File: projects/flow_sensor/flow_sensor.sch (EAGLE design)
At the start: 81 parts, among them IC1 TPS61201, IC5 REG1118

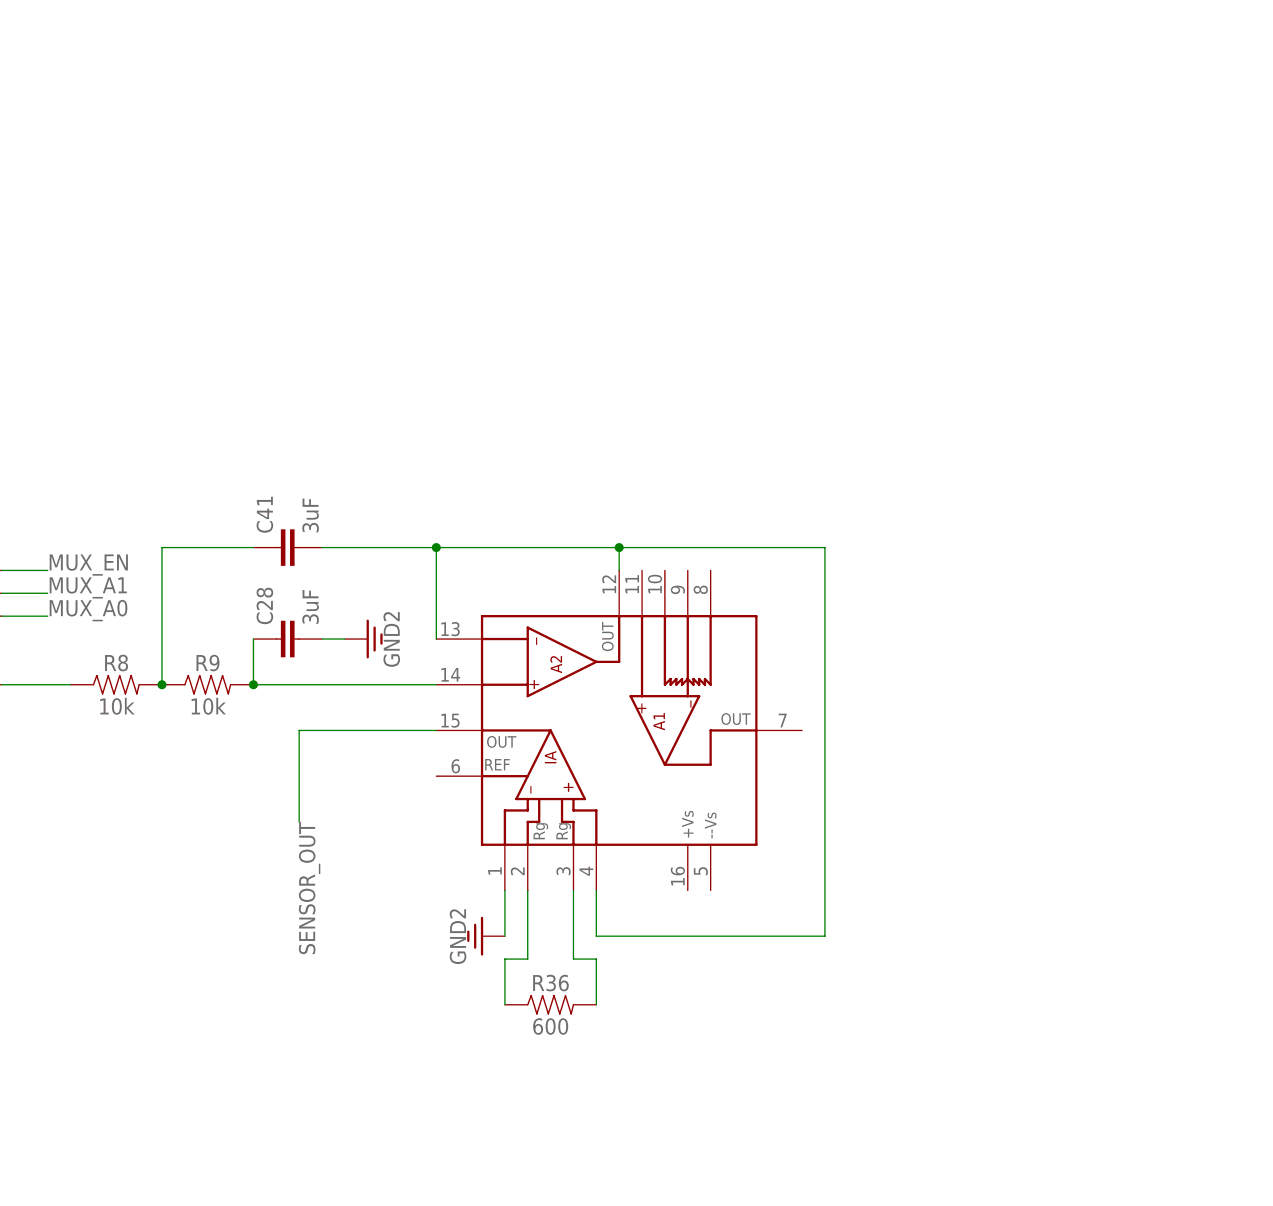
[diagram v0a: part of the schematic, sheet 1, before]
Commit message: Resubmitting work for 1/24/18
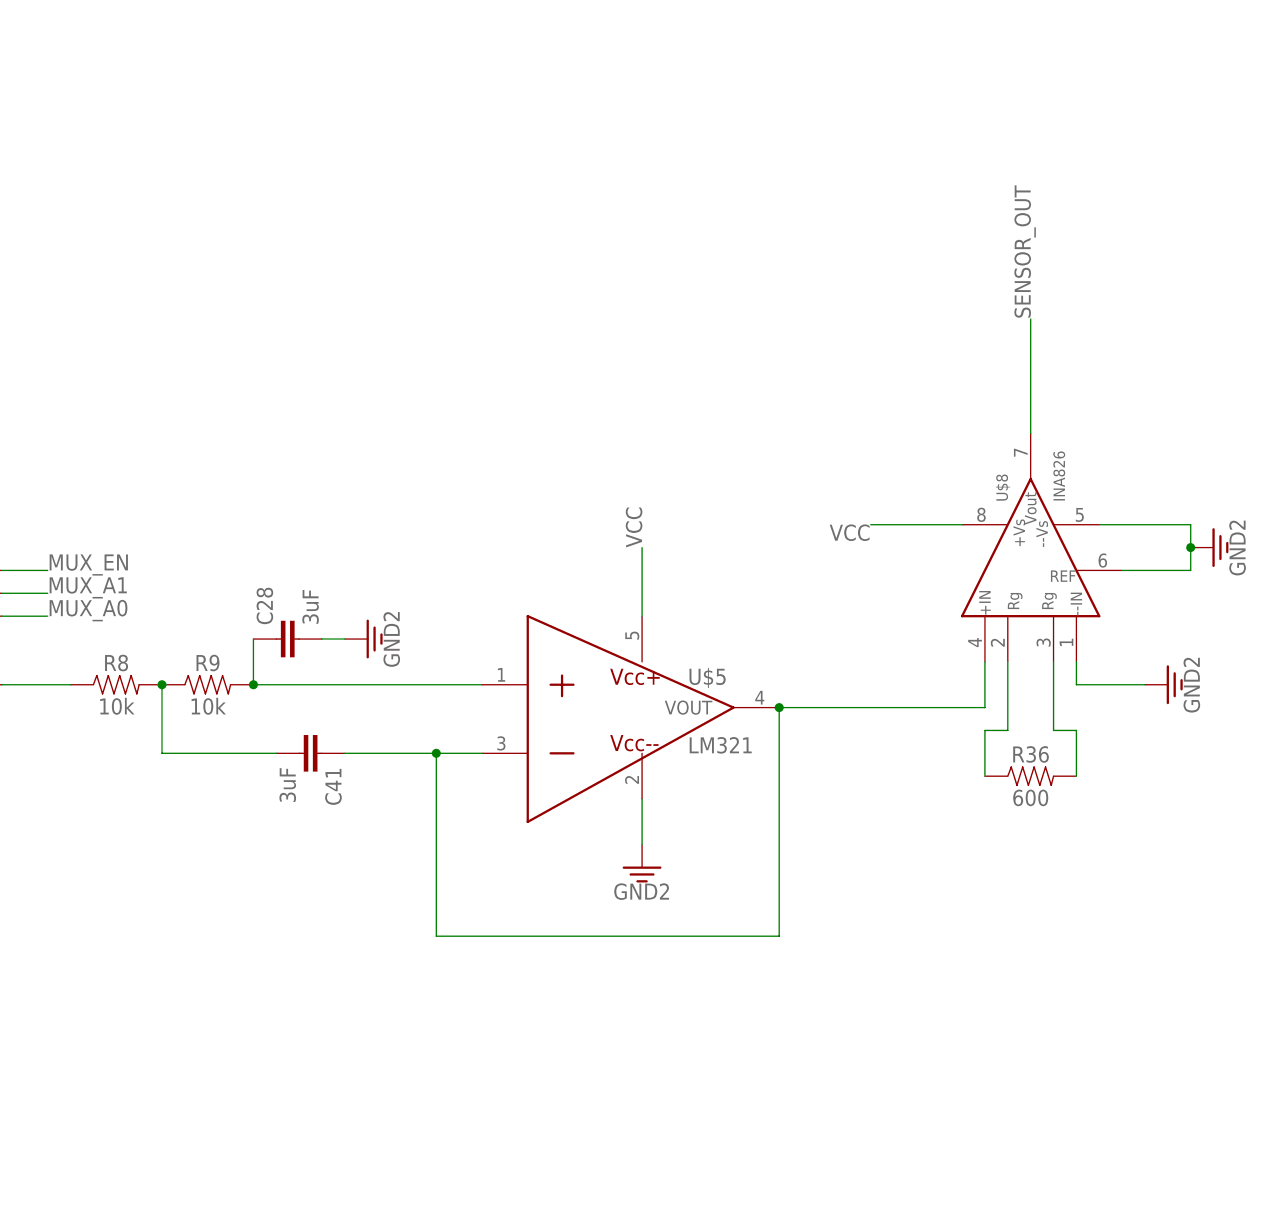
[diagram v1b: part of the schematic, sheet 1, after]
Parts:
- added U$5: LM321, my_library:LM321
- U$8: value AD8295 -> INA826; device my_library:AD8295 -> my_library:INA826
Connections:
- removed net N$35: C41.1, R8.2, R9.1
- removed net N$48: C41.2, U$8.+IN, U$8.A2-IN, U$8.A2OUT
- new net N$31: C41.1, U$5.IN-, U$5.VOUT, U$8.IN+
- new net N$36: C41.2, R8.2, R9.1
- net 3.3V: now also U$5.VCC-, U$8.IN-, U$8.REF, U$8.VS-; no longer U$8.-IN
- net N$19: now also U$5.IN+; no longer U$8.A2+IN
- net SENSOR_OUT: now also U$8.VOUT; no longer U$8.OUT
- net VCC: now also U$5.VCC+, U$8.VS+
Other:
- moved on the sheet: C41, R36
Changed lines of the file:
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@@
 <part name="U$7" library="my_library" deviceset="MAX4634" device=""/>
 <part name="GND35" library="SparkFun-PowerSymbols" deviceset="GND2" device=""/>
-<part name="U$8" library="my_library" deviceset="AD8295" device=""/>
 <part name="C41" library="SparkFun-Capacitors" deviceset="4.7UF" device="0603" value="3uF"/>
 <part name="GND36" library="SparkFun-PowerSymbols" deviceset="GND2" device=""/>
 <part name="R36" library="SparkFun-Resistors" deviceset="787OHM" device="-0603-1/10W-1%" value="600"/>
+<part name="U$5" library="my_library" deviceset="LM321" device=""/>
+<part name="GND22" library="SparkFun-PowerSymbols" deviceset="GND2" device=""/>
+<part name="U$8" library="my_library" deviceset="INA826" device=""/>
+<part name="GND28" library="SparkFun-PowerSymbols" deviceset="GND2" device=""/>
 </parts>
 <sheets>
@@
 <instance part="U$7" gate="G$1" x="254" y="5.08"/>
 <instance part="GND35" gate="G$1" x="256.54" y="27.94" rot="R180"/>
-<instance part="U$8" gate="G$1" x="337.82" y="-5.08" rot="R90"/>
-<instance part="C41" gate="G$1" x="302.26" y="15.24" rot="R90"/>
-<instance part="GND36" gate="G$1" x="322.58" y="-27.94" rot="R270"/>
-<instance part="R36" gate="G$1" x="330.2" y="-35.56"/>
+<instance part="C41" gate="G$1" x="302.26" y="-7.62" rot="R270"/>
+<instance part="GND36" gate="G$1" x="398.78" y="0" rot="R90"/>
+<instance part="R36" gate="G$1" x="383.54" y="-10.16"/>
+<instance part="U$5" gate="G$1" x="335.28" y="-2.54"/>
+<instance part="GND22" gate="G$1" x="340.36" y="-20.32"/>
+<instance part="U$8" gate="G$1" x="383.54" y="12.7" rot="R90"/>
+<instance part="GND28" gate="G$1" x="403.86" y="15.24" rot="R90"/>
 </instances>
 <busses>
@@
 <label x="251.46" y="25.4" size="1.778" layer="95" rot="R90"/>
 </segment>
+<segment>
+<wire x1="340.36" y1="7.62" x2="340.36" y2="15.24" width="0.1524" layer="91"/>
+<pinref part="U$5" gate="G$1" pin="VCC+"/>
+<label x="340.36" y="15.24" size="1.778" layer="95" rot="R90"/>
+</segment>
+<segment>
+<wire x1="375.92" y1="17.78" x2="365.76" y2="17.78" width="0.1524" layer="91"/>
+<pinref part="U$8" gate="G$1" pin="VS+"/>
+<label x="365.76" y="17.78" size="1.778" layer="95" rot="R180"/>
+</segment>
 </net>
 <net name="N$3" class="0">
@@
 </segment>
 </net>
-<net name="N$35" class="0">
-<segment>
-<pinref part="R9" gate="G$1" pin="1"/>
-<pinref part="R8" gate="G$1" pin="2"/>
-<junction x="287.02" y="0"/>
-<pinref part="C41" gate="G$1" pin="1"/>
-<wire x1="297.18" y1="15.24" x2="287.02" y2="15.24" width="0.1524" layer="91"/>
-<wire x1="287.02" y1="15.24" x2="287.02" y2="0" width="0.1524" layer="91"/>
-</segment>
-</net>
 <net name="N$19" class="0">
 <segment>
@@
 <pinref part="C28" gate="G$1" pin="1"/>
 <wire x1="297.18" y1="5.08" x2="297.18" y2="0" width="0.1524" layer="91"/>
-<wire x1="297.18" y1="0" x2="317.5" y2="0" width="0.1524" layer="91"/>
+<wire x1="297.18" y1="0" x2="322.58" y2="0" width="0.1524" layer="91"/>
 <junction x="297.18" y="0"/>
-<pinref part="U$8" gate="G$1" pin="A2+IN"/>
+<pinref part="U$5" gate="G$1" pin="IN+"/>
 </segment>
 </net>
@@
 </segment>
 <segment>
-<pinref part="U$8" gate="G$1" pin="-IN"/>
-<wire x1="325.12" y1="-22.86" x2="325.12" y2="-27.94" width="0.1524" layer="91"/>
+<pinref part="U$5" gate="G$1" pin="VCC-"/>
+<pinref part="GND22" gate="G$1" pin="3.3V"/>
+<wire x1="340.36" y1="-17.78" x2="340.36" y2="-12.7" width="0.1524" layer="91"/>
+</segment>
+<segment>
+<pinref part="U$8" gate="G$1" pin="IN-"/>
 <pinref part="GND36" gate="G$1" pin="3.3V"/>
+<wire x1="396.24" y1="0" x2="388.62" y2="0" width="0.1524" layer="91"/>
+<wire x1="388.62" y1="0" x2="388.62" y2="2.54" width="0.1524" layer="91"/>
+</segment>
+<segment>
+<pinref part="U$8" gate="G$1" pin="VS-"/>
+<pinref part="GND28" gate="G$1" pin="3.3V"/>
+<wire x1="401.32" y1="15.24" x2="401.32" y2="17.78" width="0.1524" layer="91"/>
+<wire x1="401.32" y1="17.78" x2="391.16" y2="17.78" width="0.1524" layer="91"/>
+<pinref part="U$8" gate="G$1" pin="REF"/>
+<wire x1="393.7" y1="12.7" x2="401.32" y2="12.7" width="0.1524" layer="91"/>
+<wire x1="401.32" y1="12.7" x2="401.32" y2="15.24" width="0.1524" layer="91"/>
+<junction x="401.32" y="15.24"/>
 </segment>
 </net>
@@
 </segment>
 </net>
-<net name="N$48" class="0">
-<segment>
-<pinref part="U$8" gate="G$1" pin="A2OUT"/>
-<wire x1="337.82" y1="12.7" x2="337.82" y2="15.24" width="0.1524" layer="91"/>
-<wire x1="337.82" y1="15.24" x2="317.5" y2="15.24" width="0.1524" layer="91"/>
+<net name="N$50" class="0">
+<segment>
+<pinref part="R36" gate="G$1" pin="2"/>
+<wire x1="388.62" y1="-10.16" x2="388.62" y2="-5.08" width="0.1524" layer="91"/>
+<wire x1="388.62" y1="-5.08" x2="386.08" y2="-5.08" width="0.1524" layer="91"/>
+<wire x1="386.08" y1="-5.08" x2="386.08" y2="2.54" width="0.1524" layer="91"/>
+<pinref part="U$8" gate="G$1" pin="RG'"/>
+</segment>
+</net>
+<net name="N$51" class="0">
+<segment>
+<pinref part="R36" gate="G$1" pin="1"/>
+<wire x1="378.46" y1="-10.16" x2="378.46" y2="-5.08" width="0.1524" layer="91"/>
+<wire x1="378.46" y1="-5.08" x2="381" y2="-5.08" width="0.1524" layer="91"/>
+<wire x1="381" y1="-5.08" x2="381" y2="2.54" width="0.1524" layer="91"/>
+<pinref part="U$8" gate="G$1" pin="RG"/>
+</segment>
+</net>
+<net name="SENSOR_OUT" class="0">
+<segment>
+<wire x1="383.54" y1="40.64" x2="383.54" y2="27.94" width="0.1524" layer="91"/>
+<label x="383.54" y="40.64" size="1.778" layer="95" rot="R90"/>
+<pinref part="U$8" gate="G$1" pin="VOUT"/>
+</segment>
+</net>
+<net name="N$31" class="0">
+<segment>
+<pinref part="U$5" gate="G$1" pin="VOUT"/>
+<wire x1="355.6" y1="-2.54" x2="355.6" y2="-27.94" width="0.1524" layer="91"/>
+<wire x1="355.6" y1="-27.94" x2="317.5" y2="-27.94" width="0.1524" layer="91"/>
+<pinref part="C41" gate="G$1" pin="1"/>
+<pinref part="U$5" gate="G$1" pin="IN-"/>
+<wire x1="307.34" y1="-7.62" x2="317.5" y2="-7.62" width="0.1524" layer="91"/>
+<wire x1="317.5" y1="-7.62" x2="322.58" y2="-7.62" width="0.1524" layer="91"/>
+<wire x1="317.5" y1="-27.94" x2="317.5" y2="-7.62" width="0.1524" layer="91"/>
+<junction x="317.5" y="-7.62"/>
+<wire x1="355.6" y1="-2.54" x2="378.46" y2="-2.54" width="0.1524" layer="91"/>
+<junction x="355.6" y="-2.54"/>
+<pinref part="U$8" gate="G$1" pin="IN+"/>
+<wire x1="378.46" y1="-2.54" x2="378.46" y2="2.54" width="0.1524" layer="91"/>
+</segment>
+</net>
+<net name="N$36" class="0">
+<segment>
+<pinref part="R9" gate="G$1" pin="1"/>
+<pinref part="R8" gate="G$1" pin="2"/>
+<junction x="287.02" y="0"/>
+<wire x1="287.02" y1="-7.62" x2="287.02" y2="0" width="0.1524" layer="91"/>
 <pinref part="C41" gate="G$1" pin="2"/>
-<wire x1="317.5" y1="15.24" x2="304.8" y2="15.24" width="0.1524" layer="91"/>
-<wire x1="337.82" y1="15.24" x2="360.68" y2="15.24" width="0.1524" layer="91"/>
-<wire x1="360.68" y1="15.24" x2="360.68" y2="-27.94" width="0.1524" layer="91"/>
-<junction x="337.82" y="15.24"/>
-<wire x1="360.68" y1="-27.94" x2="335.28" y2="-27.94" width="0.1524" layer="91"/>
-<pinref part="U$8" gate="G$1" pin="+IN"/>
-<wire x1="335.28" y1="-27.94" x2="335.28" y2="-22.86" width="0.1524" layer="91"/>
-<pinref part="U$8" gate="G$1" pin="A2-IN"/>
-<wire x1="317.5" y1="5.08" x2="317.5" y2="15.24" width="0.1524" layer="91"/>
-<junction x="317.5" y="15.24"/>
-</segment>
-</net>
-<net name="N$50" class="0">
-<segment>
-<pinref part="R36" gate="G$1" pin="2"/>
-<wire x1="335.28" y1="-35.56" x2="335.28" y2="-30.48" width="0.1524" layer="91"/>
-<wire x1="335.28" y1="-30.48" x2="332.74" y2="-30.48" width="0.1524" layer="91"/>
-<pinref part="U$8" gate="G$1" pin="RG'"/>
-<wire x1="332.74" y1="-30.48" x2="332.74" y2="-22.86" width="0.1524" layer="91"/>
-</segment>
-</net>
-<net name="N$51" class="0">
-<segment>
-<pinref part="R36" gate="G$1" pin="1"/>
-<wire x1="325.12" y1="-35.56" x2="325.12" y2="-30.48" width="0.1524" layer="91"/>
-<wire x1="325.12" y1="-30.48" x2="327.66" y2="-30.48" width="0.1524" layer="91"/>
-<pinref part="U$8" gate="G$1" pin="RG"/>
-<wire x1="327.66" y1="-30.48" x2="327.66" y2="-22.86" width="0.1524" layer="91"/>
-</segment>
-</net>
-<net name="SENSOR_OUT" class="0">
-<segment>
-<pinref part="U$8" gate="G$1" pin="OUT"/>
-<wire x1="317.5" y1="-5.08" x2="302.26" y2="-5.08" width="0.1524" layer="91"/>
-<wire x1="302.26" y1="-5.08" x2="302.26" y2="-15.24" width="0.1524" layer="91"/>
-<label x="302.26" y="-15.24" size="1.778" layer="95" rot="R270"/>
-</segment>
-</net>
+<wire x1="287.02" y1="-7.62" x2="299.72" y2="-7.62" width="0.1524" layer="91"/>
+</segment>
+</net>
